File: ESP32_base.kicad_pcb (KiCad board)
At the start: 2 copper layers, 112 x 54.9 mm, 32 parts, among them J1 Conn_01x16_Socket, J2 Conn_01x16_Socket, J3 Conn_01x04_Socket, J5 KH-IPEXA-SMAKWE-B080H, SW1 boot, SW2 reset, U1 ADT7310TRZ, U2 3.3V, U3 ESP32-C5-WROOM-1U-N8-R4

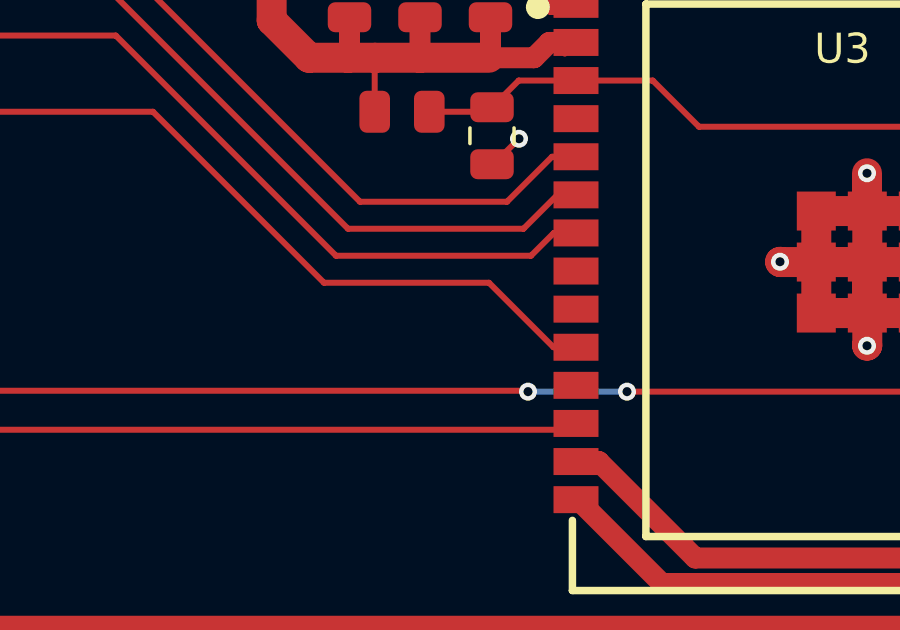
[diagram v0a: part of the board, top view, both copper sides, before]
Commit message: wip
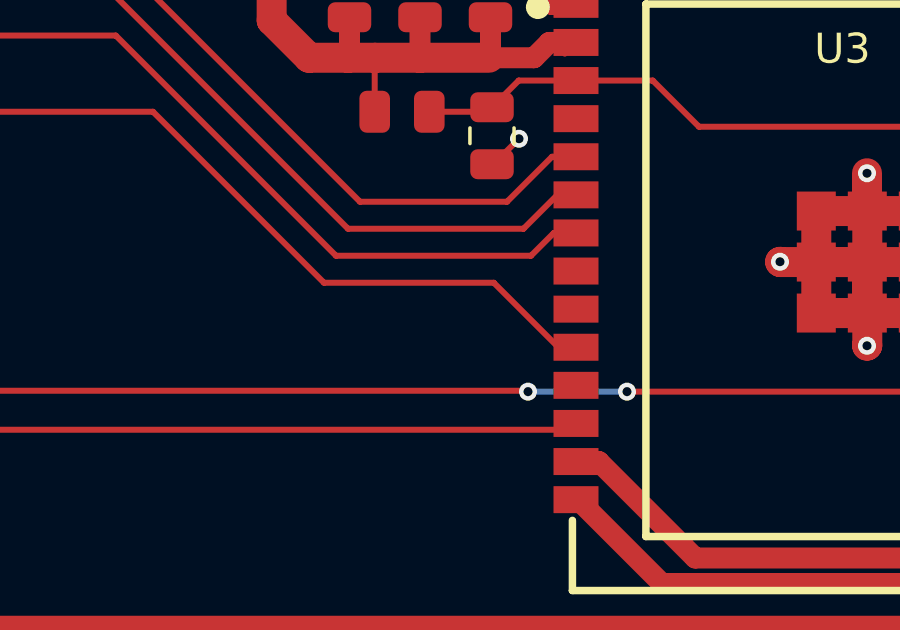
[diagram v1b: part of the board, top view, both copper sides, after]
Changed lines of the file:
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@@
 			)
 		)
-		(property "Datasheet" "~"
+		(property "Datasheet" "https://www.lcsc.com/datasheet/C2905421.pdf"
 			(at 0 0 0)
 			(layer "F.Fab")
@@
 			)
 		)
-		(property "Description" "Generic connector, single row, 01x16, script generated"
+		(property "Description" "Female Header 16 Position 2.54mm Pitch Single Row Through Hole -40℃~+105℃"
 			(at 0 0 0)
 			(layer "F.Fab")
@@
 			)
 		)
+		(property "Part" "KH-2.54FH-1X16P-H8.5"
+			(at 0 0 0)
+			(unlocked yes)
+			(layer "F.Fab")
+			(hide yes)
+			(effects
+				(font
+					(size 1 1)
+					(thickness 0.15)
+				)
+			)
+		)
 		(property ki_fp_filters "Connector*:*_1x??_*")
 		(sheetname "/")
@@
 			)
 		)
-		(property "Datasheet" "~"
+		(property "Datasheet" "https://www.lcsc.com/datasheet/C2905421.pdf"
 			(at 0 0 0)
 			(layer "F.Fab")
@@
 			)
 		)
-		(property "Description" "Generic connector, single row, 01x16, script generated"
+		(property "Description" "Female Header 16 Position 2.54mm Pitch Single Row Through Hole -40℃~+105℃"
 			(at 0 0 0)
 			(layer "F.Fab")
@@
 			)
 		)
+		(property "Part" "KH-2.54FH-1X16P-H8.5"
+			(at 0 0 0)
+			(unlocked yes)
+			(layer "F.Fab")
+			(hide yes)
+			(effects
+				(font
+					(size 1 1)
+					(thickness 0.15)
+				)
+			)
+		)
 		(property ki_fp_filters "Connector*:*_1x??_*")
 		(sheetname "/")
@@
 	)
 	(segment
-		(start 122.3 234.5)
-		(end 127.8 234.5)
+		(start 104.1 228.8)
+		(end 116.6 228.8)
 		(width 0.2)
 		(layer "F.Cu")
@@
 	)
 	(segment
-		(start 104.1 228.8)
-		(end 116.6 228.8)
+		(start 122.3 234.5)
+		(end 127.96 234.5)
 		(width 0.2)
 		(layer "F.Cu")
@@
 	)
 	(segment
-		(start 127.8 234.5)
-		(end 129.95 236.65)
+		(start 91.52 228.8)
+		(end 87.0186 228.8)
 		(width 0.2)
 		(layer "F.Cu")
@@
 	)
 	(segment
-		(start 129.95 236.65)
-		(end 130.7 236.65)
+		(start 127.96 234.5)
+		(end 130.11 236.65)
 		(width 0.2)
 		(layer "F.Cu")
@@
 	)
 	(segment
-		(start 116.6 228.8)
-		(end 122.3 234.5)
+		(start 130.11 236.65)
+		(end 130.7 236.65)
 		(width 0.2)
 		(layer "F.Cu")
@@
 	)
 	(segment
-		(start 91.52 228.8)
-		(end 87.0186 228.8)
+		(start 116.6 228.8)
+		(end 122.3 234.5)
 		(width 0.2)
 		(layer "F.Cu")
